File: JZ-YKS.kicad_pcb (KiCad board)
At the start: 2 copper layers, 50 x 50 mm, 55 parts, among them IC1 JZ4725, J1 USB_MINIB, U1 PINHEAD30, U2 PINHEAD30, U3 VREG-DUAL, U4 HY27UG088G5M, U5 P3V56S40ETP-G6, X1 32768Hz, X2 12MHz

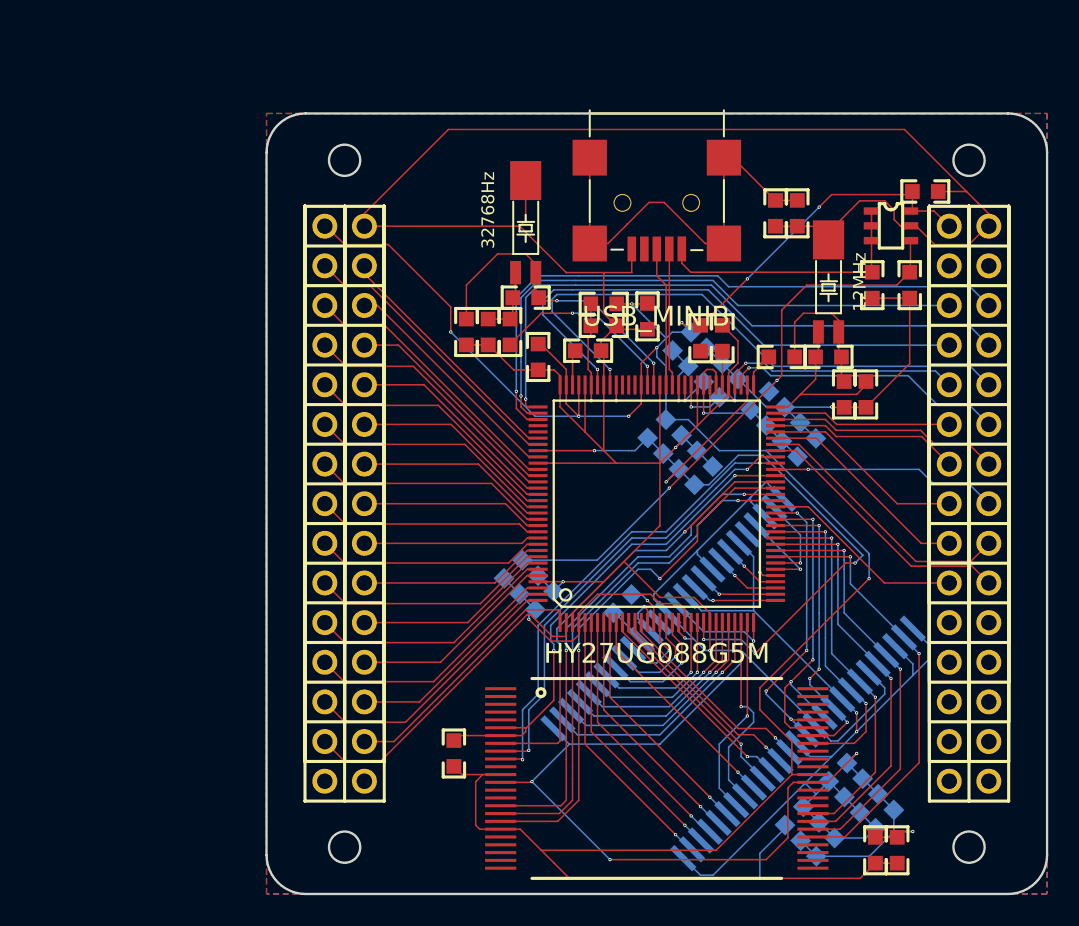
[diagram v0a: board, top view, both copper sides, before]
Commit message: that fucking TSOP library is all wrong
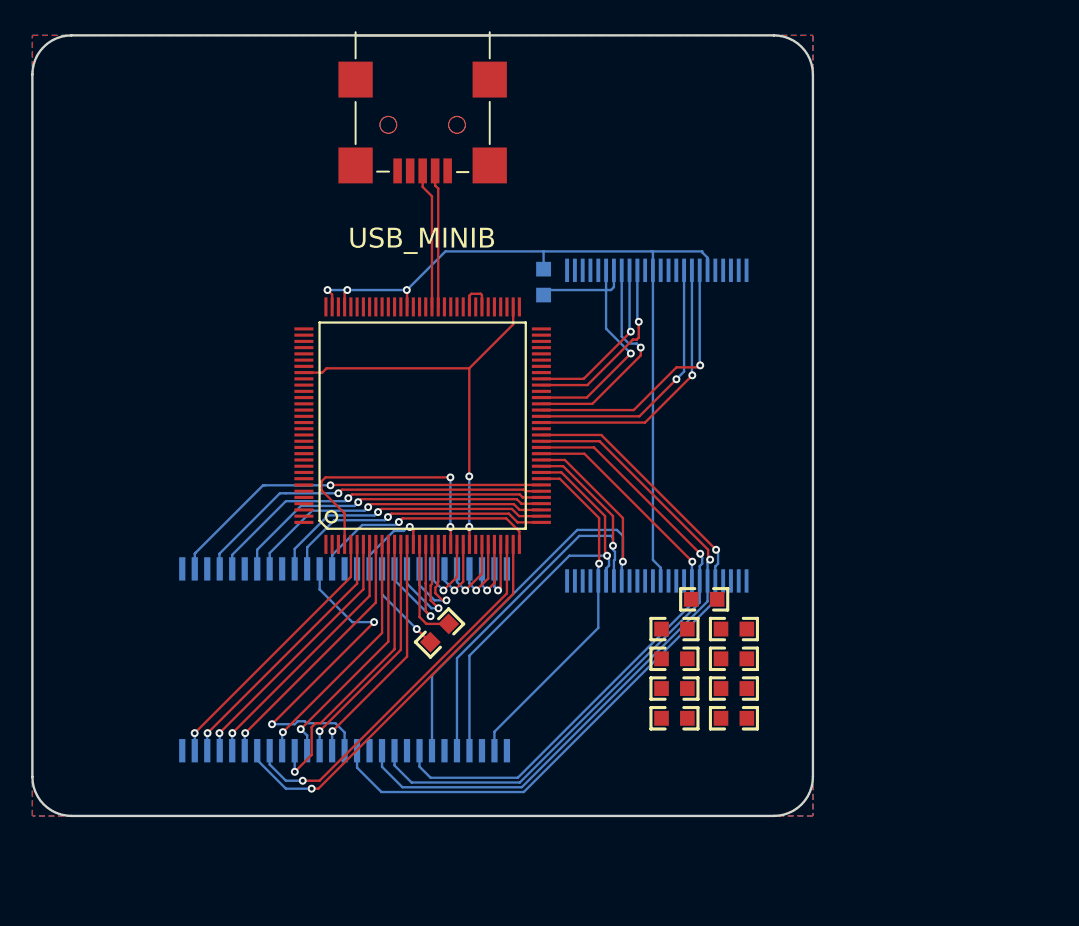
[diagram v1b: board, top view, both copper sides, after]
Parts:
- removed C1, C13, C3, C4, C5, C9: 0.1uF, size-0603
- removed C10, C7, C8: 1uF, size-0603
- removed C11, C12: 0.01uF, size-0603
- removed C14, C15, C2, C6: 10uF, size-0603
- removed C16, C17, C18, C19: 22pF, size-0603
- removed C20, C29, C30, C31: C, size-0603
- removed FB1, FB2, FB3, FB5, FB6, FB7, FB8: BKP1608HS121, size-0603
- removed R1: 10k, size-0603
- removed R2, R3: 33, size-0603
- removed R4: 10M, size-0603
- removed R5: 1M, size-0603
- removed U1, U2: PINHEAD30, PINHEAD30
- removed U3: VREG-DUAL, sot23-6
- removed X1: 32768Hz, crystal
- removed X2: 12MHz, crystal
- C21, C22, C23, C24, C25, C26, FB9, R6: moved to F.Cu
- R7: moved to B.Cu
- U4: footprint TSOP48 -> tsop48; moved to B.Cu
- U5: footprint TSOP54 -> tsop54
- moved U5 36.5 mm to (130.0, 115.0), turned to 180 degrees
- moved R7 30.7 mm to (142.7, 90.8), turned to 270 degrees
- moved U4 22.6 mm to (150.0, 100.0), turned to 0 degrees
- moved C28 20.1 mm to (151.1, 113.0), turned to 180 degrees
- moved C27 17.8 mm to (151.1, 114.9), turned to 180 degrees
- moved IC1 15.8 mm to (135.0, 100.0)
- moved J1 15.8 mm to (135.0, 75.0)
- moved FB9 15.0 mm to (153.0, 111.1), turned to 180 degrees
- moved C26 14.0 mm to (151.1, 116.8), turned to 180 degrees
- moved R6 11.9 mm to (136.1, 113.3)
- moved C24 11.6 mm to (154.9, 118.7), turned to 0 degrees
- moved C23 11.4 mm to (154.9, 116.8), turned to 0 degrees
- moved C21 11.3 mm to (154.9, 113.0), turned to 0 degrees
- moved C25 11.3 mm to (151.1, 118.7), turned to 180 degrees
- moved C22 11.3 mm to (154.9, 114.9), turned to 0 degrees
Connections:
- J1 pad 6: N-0000081 -> GND
- J1 pad 7: N-0000081 -> GND
- J1 pad 8: N-0000081 -> GND
- J1 pad 9: N-0000081 -> GND
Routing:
- net GND: track 312.3 -> 0.00 mm, vias 10 -> 0
- net +3.3V: track 167.8 -> 52.4 mm, vias 10 -> 3
- net N-00000159: track 62.6 -> 21.1 mm
- net MIC: track 40.4 -> 0.00 mm, vias 1 -> 0
- net IN_L: track 39.3 -> 0.00 mm, vias 1 -> 0
- net +1.8V: track 37.9 -> 0.00 mm, vias 2 -> 0
- net HP_R: track 37.5 -> 0.00 mm, vias 1 -> 0
- net IN_R: track 36.8 -> 0.00 mm, vias 1 -> 0
- net HP_L: track 34.6 -> 0.00 mm, vias 1 -> 0
- net D7: track 19.4 -> 47.4 mm, vias 4 -> 1
- net N-0000081: track 27.6 -> 0.00 mm
- net D6: track 21.3 -> 44.4 mm, vias 3 -> 1
- net D5: track 19.2 -> 42.0 mm, vias 4 -> 1
- net N-00000101: track 49.6 -> 27.1 mm, vias 5 -> 2
- net PCLK: track 21.4 -> 0.00 mm
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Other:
- outline, holes or cut-outs redrawn
- net class Default: clearance 0.1 -> 0.1524; trace_width 0.1 -> 0.1524; via_dia 0.21 -> 0.508; via_drill 0.2 -> 0.3302
- net class Power added: clearance 0.3048, trace_width 0.3048, via_dia 0.508, via_drill 0.3302
- rule trace_clearance: 0.1 -> 0.1524
- rule trace_min: 0.1 -> 0.1524
- rule via_min_drill: 0.2 -> 0.3302
- rule via_min_size: 0.21 -> 0.508
